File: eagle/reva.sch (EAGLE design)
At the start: 233 parts, among them IC1 LM555D, IC2 74HC174D, J1 TYPE-C-31-M-12, U1 TPS63000DRCR

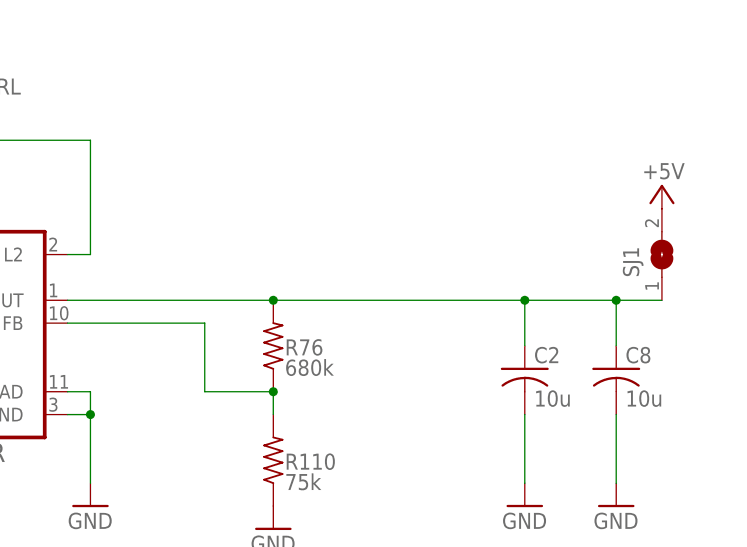
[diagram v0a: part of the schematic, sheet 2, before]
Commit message: Save
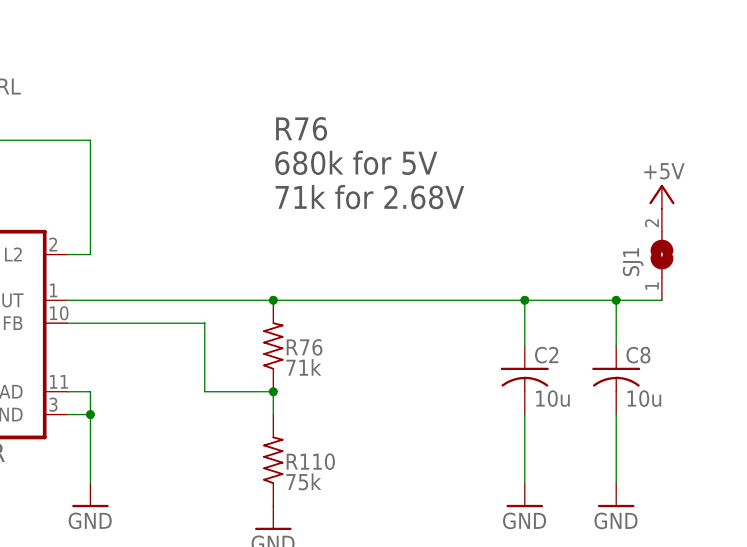
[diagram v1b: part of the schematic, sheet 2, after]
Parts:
- R76: value 680k -> 71k
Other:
- note added: "R76 680k for 5V 71k for 2.68V"
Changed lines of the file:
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@@
 <part name="H4" library="holes" library_urn="urn:adsk.eagle:library:237" deviceset="MOUNT-HOLE" device="3.3" package3d_urn="urn:adsk.eagle:package:14278/1"/>
 <part name="BAT1" library="flashing_ece_2025" deviceset="CR2450" device=""/>
-<part name="R76" library="adafruit" deviceset="R-US_" device="R0603" value="680k"/>
+<part name="R76" library="adafruit" deviceset="R-US_" device="R0603" value="71k"/>
 <part name="R110" library="adafruit" deviceset="R-US_" device="R0603" value="75k"/>
 <part name="GND24" library="supply1" library_urn="urn:adsk.eagle:library:371" deviceset="GND" device=""/>
@@
 <text x="302.26" y="10.16" size="6.4516" layer="94">PWR</text>
 <text x="215.9" y="93.98" size="2.54" layer="97">R76 = R110 * ((Vout/0.5)-1)</text>
+<text x="274.32" y="147.32" size="2.54" layer="97">R76
+680k for 5V
+71k for 2.68V</text>
 </plain>
 <instances>
@@
 </drawing>
 <compatibility>
+<note version="6.3" minversion="6.2.2" severity="warning">
+Since Version 6.2.2 text objects can contain more than one line,
+which will not be processed correctly with this version.
+</note>
 <note version="8.2" severity="warning">
 Since Version 8.2, EAGLE supports online libraries. The ids
